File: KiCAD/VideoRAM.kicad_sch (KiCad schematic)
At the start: 10 parts

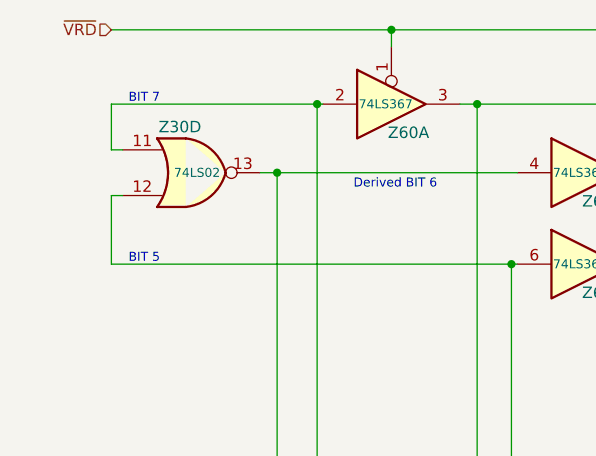
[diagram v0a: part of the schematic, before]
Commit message: Update to V9
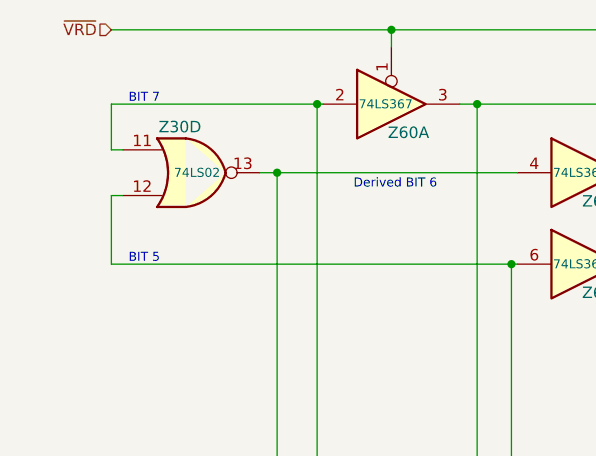
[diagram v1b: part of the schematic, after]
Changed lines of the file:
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@@
 (kicad_sch
-	(version 20231120)
+	(version 20250114)
 	(generator "eeschema")
-	(generator_version "8.0")
+	(generator_version "9.0")
 	(paper "USLetter")
 	(title_block
@@
 		(comment 4 "Video RAM & Gating")
 	)
+	(text "Derived BIT 6"
+		(exclude_from_sim no)
+		(at 79.375 37.465 0)
+		(effects
+			(font
+				(size 1 1)
+			)
+			(justify right bottom)
+		)
+	)
+	(text "BIT 5"
+		(exclude_from_sim no)
+		(at 45.085 45.72 0)
+		(effects
+			(font
+				(size 1 1)
+			)
+			(justify left bottom)
+		)
+	)
+	(text "BIT 7"
+		(exclude_from_sim no)
+		(at 45.085 27.94 0)
+		(effects
+			(font
+				(size 1 1)
+			)
+			(justify left bottom)
+		)
+	)
 	(junction
 		(at 156.21 116.205)
@@
 		)
 	)
-	(text "Derived BIT 6"
-		(exclude_from_sim no)
-		(at 79.375 37.465 0)
-		(effects
-			(font
-				(size 1 1)
-			)
-			(justify right bottom)
-		)
-	)
-	(text "BIT 5"
-		(exclude_from_sim no)
-		(at 45.085 45.72 0)
-		(effects
-			(font
-				(size 1 1)
-			)
-			(justify left bottom)
-		)
-	)
-	(text "BIT 7"
-		(exclude_from_sim no)
-		(at 45.085 27.94 0)
-		(effects
-			(font
-				(size 1 1)
-			)
-			(justify left bottom)
-		)
-	)
 	(label "D1"
 		(at 222.885 63.5 180)
-		(fields_autoplaced yes)
 		(effects
 			(font
@@
 	(label "VA2"
 		(at 55.88 93.345 0)
-		(fields_autoplaced yes)
 		(effects
 			(font
@@
 	(label "D2"
 		(at 222.885 59.055 180)
-		(fields_autoplaced yes)
 		(effects
 			(font
@@
 	(label "VA5"
 		(at 55.88 100.965 0)
-		(fields_autoplaced yes)
 		(effects
 			(font
@@
 	(label "D3"
 		(at 222.885 54.61 180)
-		(fields_autoplaced yes)
 		(effects
 			(font
@@
 	(label "D0"
 		(at 222.885 67.945 180)
-		(fields_autoplaced yes)
 		(effects
 			(font
@@
 	(label "VA9"
 		(at 55.88 111.125 0)
-		(fields_autoplaced yes)
 		(effects
 			(font
@@
 	(label "D5"
 		(at 222.885 45.72 180)
-		(fields_autoplaced yes)
 		(effects
 			(font
@@
 	(label "VA4"
 		(at 55.88 98.425 0)
-		(fields_autoplaced yes)
 		(effects
 			(font
@@
 	(label "VA1"
 		(at 55.88 90.805 0)
-		(fields_autoplaced yes)
 		(effects
 			(font
@@
 	(label "VD5"
 		(at 219.075 156.21 0)
-		(fields_autoplaced yes)
 		(effects
 			(font
@@
 	(label "D4"
 		(at 222.885 50.165 180)
-		(fields_autoplaced yes)
 		(effects
 			(font
@@
 	(label "VD0"
 		(at 219.075 143.51 0)
-		(fields_autoplaced yes)
 		(effects
 			(font
@@
 	(label "VD1"
 		(at 219.075 146.05 0)
-		(fields_autoplaced yes)
 		(effects
 			(font
@@
 	(label "VA7"
 		(at 55.88 106.045 0)
-		(fields_autoplaced yes)
 		(effects
 			(font
@@
 	(label "D6"
 		(at 222.885 35.56 180)
-		(fields_autoplaced yes)
 		(effects
 			(font
@@
 	(label "VA3"
 		(at 55.88 95.885 0)
-		(fields_autoplaced yes)
 		(effects
 			(font
@@
 	(label "VD2"
 		(at 219.075 148.59 0)
-		(fields_autoplaced yes)
 		(effects
 			(font
@@
 	(label "VD3"
 		(at 219.075 151.13 0)
-		(fields_autoplaced yes)
 		(effects
 			(font
@@
 	(label "VD4"
 		(at 219.075 153.67 0)
-		(fields_autoplaced yes)
 		(effects
 			(font
@@
 	(label "VA6"
 		(at 55.88 103.505 0)
-		(fields_autoplaced yes)
 		(effects
 			(font
@@
 	(label "D7"
 		(at 222.885 27.94 180)
-		(fields_autoplaced yes)
 		(effects
 			(font
@@
 	(label "VA8"
 		(at 55.88 108.585 0)
-		(fields_autoplaced yes)
 		(effects
 			(font
@@
 	(label "VA0"
 		(at 55.88 88.265 0)
-		(fields_autoplaced yes)
 		(effects
 			(font
@@
 	(label "VD6"
 		(at 219.075 158.75 0)
-		(fields_autoplaced yes)
 		(effects
 			(font
@@
 	(label "VD7"
 		(at 219.075 161.29 0)
-		(fields_autoplaced yes)
 		(effects
 			(font
@@
 		(shape input)
 		(at 43.18 116.205 180)
-		(fields_autoplaced yes)
 		(effects
 			(font
@@
 		(shape bidirectional)
 		(at 228.6 24.13 0)
-		(fields_autoplaced yes)
 		(effects
 			(font
@@
 		(shape input)
 		(at 50.165 84.455 180)
-		(fields_autoplaced yes)
 		(effects
 			(font
@@
 		(shape input)
 		(at 43.18 19.685 180)
-		(fields_autoplaced yes)
 		(effects
 			(font
@@
 		(shape output)
 		(at 227.965 139.7 0)
-		(fields_autoplaced yes)
-		(effects
-			(font
+		(effects
+			(font
